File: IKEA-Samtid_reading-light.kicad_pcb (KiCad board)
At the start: 2 copper layers, 21 x 100 mm, 30 parts, among them IC1 ATTINY25-S, P1 CONN_2, U1 MCP1804-SOT23-5, U2 PT4115-SOT89-5

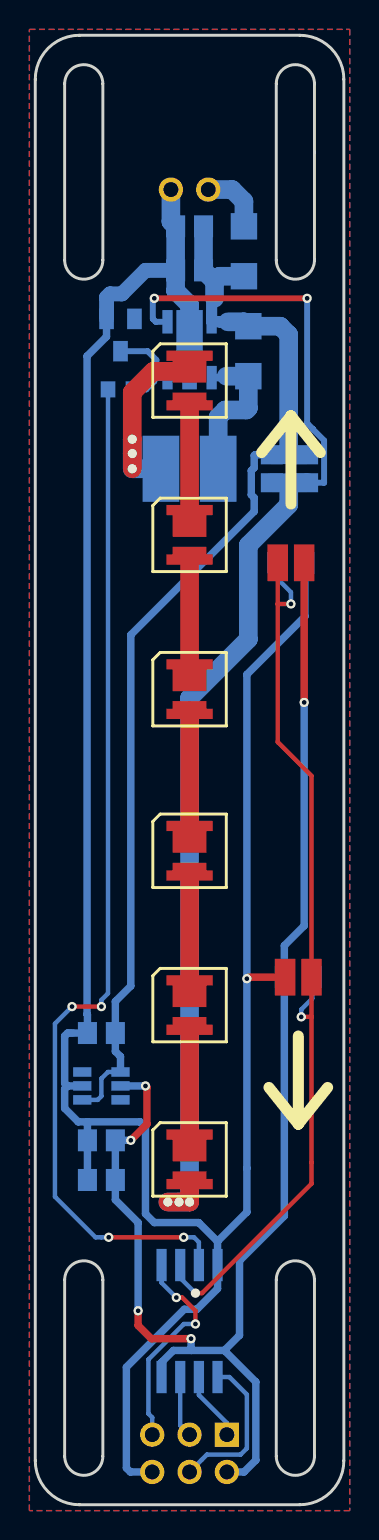
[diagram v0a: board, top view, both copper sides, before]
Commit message: Tweaks.
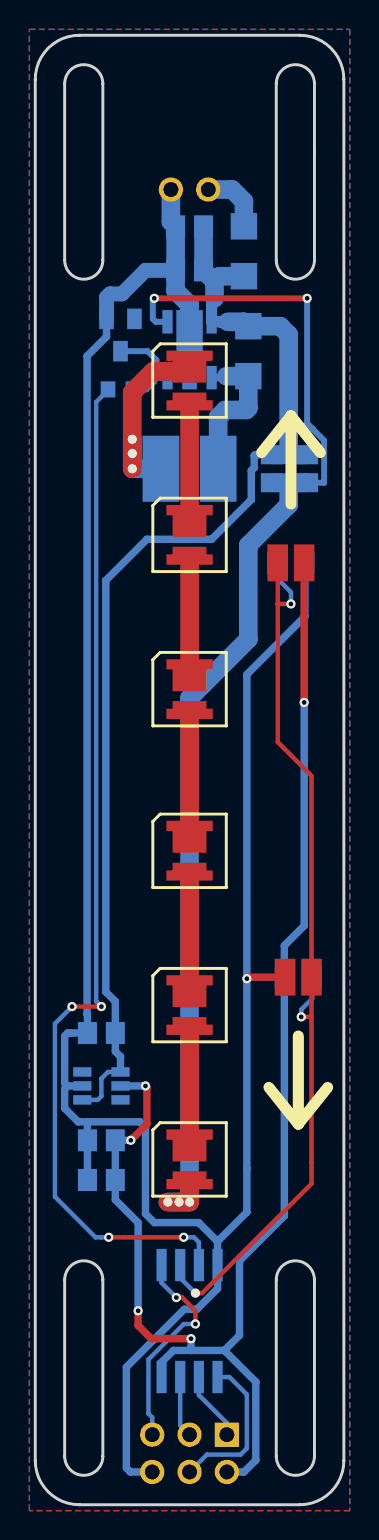
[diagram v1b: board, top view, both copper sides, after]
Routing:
- net +24V: track 76.8 -> 79.7 mm
